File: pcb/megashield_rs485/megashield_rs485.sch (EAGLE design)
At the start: 21 parts, among them J11 DYNAMIXEL_RS485, U1 RS485

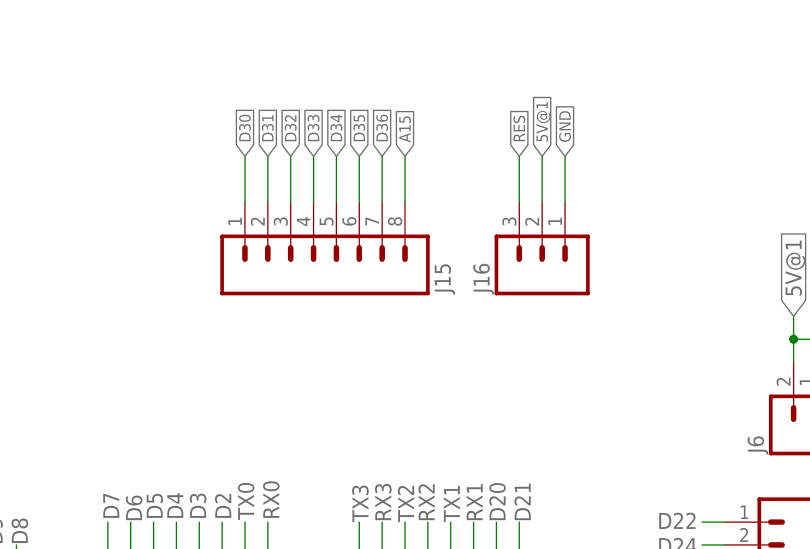
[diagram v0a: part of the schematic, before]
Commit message: PCB with LCD
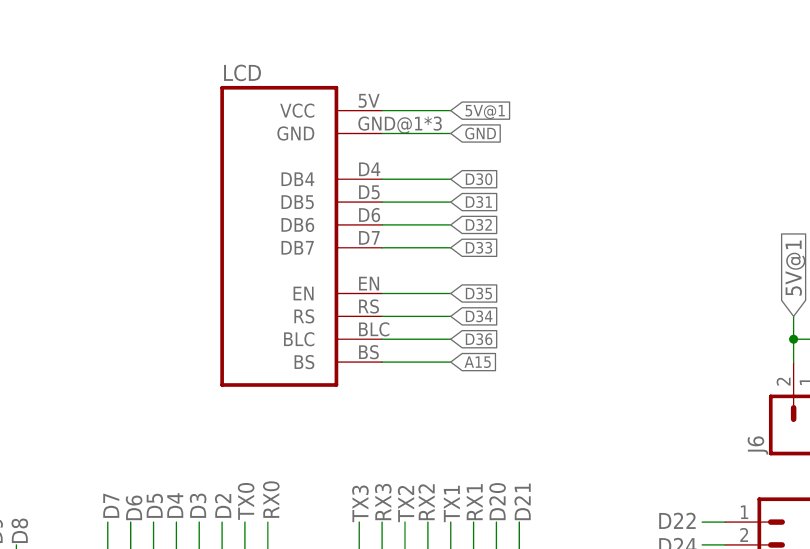
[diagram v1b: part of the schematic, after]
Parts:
- removed J15: (no value), mecatronica_eagle_lib:M08LONGPADS
- removed J16: (no value), mecatronica_eagle_lib:M03LONGPADS
- added LCD: LCD_SHIELD, mecatronica_eagle_lib:LCD_SHIELD
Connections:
- net 5V@1: now also LCD.VCC; no longer J16.2
- net A15: now also LCD.BS; no longer J15.8
- net D30: now also LCD.DB4; no longer J15.1
- net D31: now also LCD.DB5; no longer J15.2
- net D32: now also LCD.DB6; no longer J15.3
- net D33: now also LCD.DB7; no longer J15.4
- net D34: now also LCD.RS; no longer J15.5
- net D35: now also LCD.EN; no longer J15.6
- net D36: now also LCD.BLC; no longer J15.7
- net GND: now also LCD.GND; no longer J16.1
- net RES: no longer J16.3
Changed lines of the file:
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@@
 <?xml version="1.0" encoding="utf-8"?>
 <!DOCTYPE eagle SYSTEM "eagle.dtd">
-<eagle version="7.4.0">
+<eagle version="7.6.0">
 <drawing>
 <settings>
@@
 <setting verticaltext="up"/>
 </settings>
-<grid distance="0.1" unitdist="inch" unit="inch" style="lines" multiple="1" display="yes" altdistance="0.01" altunitdist="inch" altunit="inch"/>
+<grid distance="0.1" unitdist="inch" unit="inch" style="lines" multiple="1" display="no" altdistance="0.01" altunitdist="inch" altunit="inch"/>
 <layers>
 <layer number="1" name="Top" color="4" fill="1" visible="no" active="no"/>
@@
 <layer number="230" name="230bmp" color="7" fill="1" visible="yes" active="yes"/>
 <layer number="231" name="231bmp" color="7" fill="1" visible="yes" active="yes"/>
+<layer number="232" name="Eagle3D_PG2" color="7" fill="1" visible="no" active="no"/>
+<layer number="233" name="Eagle3D_PG3" color="7" fill="1" visible="no" active="no"/>
 <layer number="248" name="Housing" color="7" fill="1" visible="yes" active="yes"/>
 <layer number="249" name="Edge" color="7" fill="1" visible="yes" active="yes"/>
@@
 <part name="R2" library="mecatronica_eagle_lib" deviceset="RESISTOR" device="PTH-1/4W" value="10k"/>
 <part name="GND5" library="SparkFun" deviceset="GND" device=""/>
-<part name="J15" library="mecatronica_eagle_lib" deviceset="M08" device="LONGPADS"/>
-<part name="J16" library="mecatronica_eagle_lib" deviceset="M03" device="LONGPADS"/>
+<part name="LCD" library="mecatronica_eagle_lib" deviceset="LCD_SHIELD" device=""/>
 </parts>
 <sheets>
@@
 <instance part="R2" gate="G$1" x="30.48" y="165.1" rot="R90"/>
 <instance part="GND5" gate="1" x="104.14" y="134.62"/>
-<instance part="J15" gate="G$1" x="160.02" y="154.94" rot="MR90"/>
-<instance part="J16" gate="J$1" x="185.42" y="152.4" rot="R90"/>
+<instance part="LCD" gate="G$1" x="154.94" y="157.48"/>
 </instances>
 <busses>
@@
 <label x="83.82" y="57.15" size="1.778" layer="95" rot="R90"/>
 <pinref part="J10" gate="G$1" pin="1"/>
-</segment>
-<segment>
-<pinref part="J16" gate="J$1" pin="3"/>
-<wire x1="182.88" y1="160.02" x2="182.88" y2="165.1" width="0.1524" layer="91"/>
-<label x="182.88" y="165.1" size="1.27" layer="95" rot="R90" xref="yes"/>
 </segment>
 </net>
@@
 </segment>
 <segment>
-<pinref part="J15" gate="G$1" pin="8"/>
-<wire x1="170.18" y1="160.02" x2="170.18" y2="165.1" width="0.1524" layer="91"/>
-<label x="170.18" y="165.1" size="1.27" layer="95" rot="R90" xref="yes"/>
+<wire x1="167.64" y1="142.24" x2="175.26" y2="142.24" width="0.1524" layer="91"/>
+<label x="175.26" y="142.24" size="1.27" layer="95" xref="yes"/>
+<pinref part="LCD" gate="G$1" pin="BS"/>
 </segment>
 </net>
@@
 </segment>
 <segment>
-<pinref part="J15" gate="G$1" pin="1"/>
-<wire x1="152.4" y1="160.02" x2="152.4" y2="165.1" width="0.1524" layer="91"/>
-<label x="152.4" y="165.1" size="1.27" layer="95" rot="R90" xref="yes"/>
+<wire x1="167.64" y1="162.56" x2="175.26" y2="162.56" width="0.1524" layer="91"/>
+<label x="175.26" y="162.56" size="1.27" layer="95" xref="yes"/>
+<pinref part="LCD" gate="G$1" pin="DB4"/>
 </segment>
 </net>
@@
 </segment>
 <segment>
-<pinref part="J15" gate="G$1" pin="3"/>
-<wire x1="157.48" y1="160.02" x2="157.48" y2="165.1" width="0.1524" layer="91"/>
-<label x="157.48" y="165.1" size="1.27" layer="95" rot="R90" xref="yes"/>
+<wire x1="167.64" y1="157.48" x2="175.26" y2="157.48" width="0.1524" layer="91"/>
+<label x="175.26" y="157.48" size="1.27" layer="95" xref="yes"/>
+<pinref part="LCD" gate="G$1" pin="DB6"/>
 </segment>
 </net>
@@
 </segment>
 <segment>
-<pinref part="J15" gate="G$1" pin="5"/>
-<wire x1="162.56" y1="160.02" x2="162.56" y2="165.1" width="0.1524" layer="91"/>
-<label x="162.56" y="165.1" size="1.27" layer="95" rot="R90" xref="yes"/>
+<wire x1="167.64" y1="147.32" x2="175.26" y2="147.32" width="0.1524" layer="91"/>
+<label x="175.26" y="147.32" size="1.27" layer="95" xref="yes"/>
+<pinref part="LCD" gate="G$1" pin="RS"/>
 </segment>
 </net>
@@
 </segment>
 <segment>
-<pinref part="J15" gate="G$1" pin="7"/>
-<wire x1="167.64" y1="160.02" x2="167.64" y2="165.1" width="0.1524" layer="91"/>
-<label x="167.64" y="165.1" size="1.27" layer="95" rot="R90" xref="yes"/>
+<wire x1="167.64" y1="144.78" x2="175.26" y2="144.78" width="0.1524" layer="91"/>
+<label x="175.26" y="144.78" size="1.27" layer="95" xref="yes"/>
+<pinref part="LCD" gate="G$1" pin="BLC"/>
 </segment>
 </net>
@@
 </segment>
 <segment>
-<pinref part="J15" gate="G$1" pin="2"/>
-<wire x1="154.94" y1="160.02" x2="154.94" y2="165.1" width="0.1524" layer="91"/>
-<label x="154.94" y="165.1" size="1.27" layer="95" rot="R90" xref="yes"/>
+<wire x1="167.64" y1="160.02" x2="175.26" y2="160.02" width="0.1524" layer="91"/>
+<label x="175.26" y="160.02" size="1.27" layer="95" xref="yes"/>
+<pinref part="LCD" gate="G$1" pin="DB5"/>
 </segment>
 </net>
@@
 </segment>
 <segment>
-<pinref part="J15" gate="G$1" pin="4"/>
-<wire x1="160.02" y1="160.02" x2="160.02" y2="165.1" width="0.1524" layer="91"/>
-<label x="160.02" y="165.1" size="1.27" layer="95" rot="R90" xref="yes"/>
+<wire x1="167.64" y1="154.94" x2="175.26" y2="154.94" width="0.1524" layer="91"/>
+<label x="175.26" y="154.94" size="1.27" layer="95" xref="yes"/>
+<pinref part="LCD" gate="G$1" pin="DB7"/>
 </segment>
 </net>
@@
 </segment>
 <segment>
-<pinref part="J15" gate="G$1" pin="6"/>
-<wire x1="165.1" y1="160.02" x2="165.1" y2="165.1" width="0.1524" layer="91"/>
-<label x="165.1" y="165.1" size="1.27" layer="95" rot="R90" xref="yes"/>
+<wire x1="167.64" y1="149.86" x2="175.26" y2="149.86" width="0.1524" layer="91"/>
+<label x="175.26" y="149.86" size="1.27" layer="95" xref="yes"/>
+<pinref part="LCD" gate="G$1" pin="EN"/>
 </segment>
 </net>
@@
 </segment>
 <segment>
-<pinref part="J16" gate="J$1" pin="1"/>
-<wire x1="187.96" y1="160.02" x2="187.96" y2="165.1" width="0.1524" layer="91"/>
-<label x="187.96" y="165.1" size="1.27" layer="95" rot="R90" xref="yes"/>
+<wire x1="167.64" y1="167.64" x2="175.26" y2="167.64" width="0.1524" layer="91"/>
+<label x="175.26" y="167.64" size="1.27" layer="95" xref="yes"/>
+<pinref part="LCD" gate="G$1" pin="GND"/>
 </segment>
 </net>
@@
 </segment>
 <segment>
-<pinref part="J16" gate="J$1" pin="2"/>
-<wire x1="185.42" y1="160.02" x2="185.42" y2="165.1" width="0.1524" layer="91"/>
-<label x="185.42" y="165.1" size="1.27" layer="95" rot="R90" xref="yes"/>
-</segment>
-</net>
+<wire x1="167.64" y1="170.18" x2="175.26" y2="170.18" width="0.1524" layer="91"/>
+<label x="175.26" y="170.18" size="1.27" layer="95" xref="yes"/>
+<pinref part="LCD" gate="G$1" pin="VCC"/>
+</segment>
+</net>
